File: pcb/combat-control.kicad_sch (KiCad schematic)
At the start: 0 parts

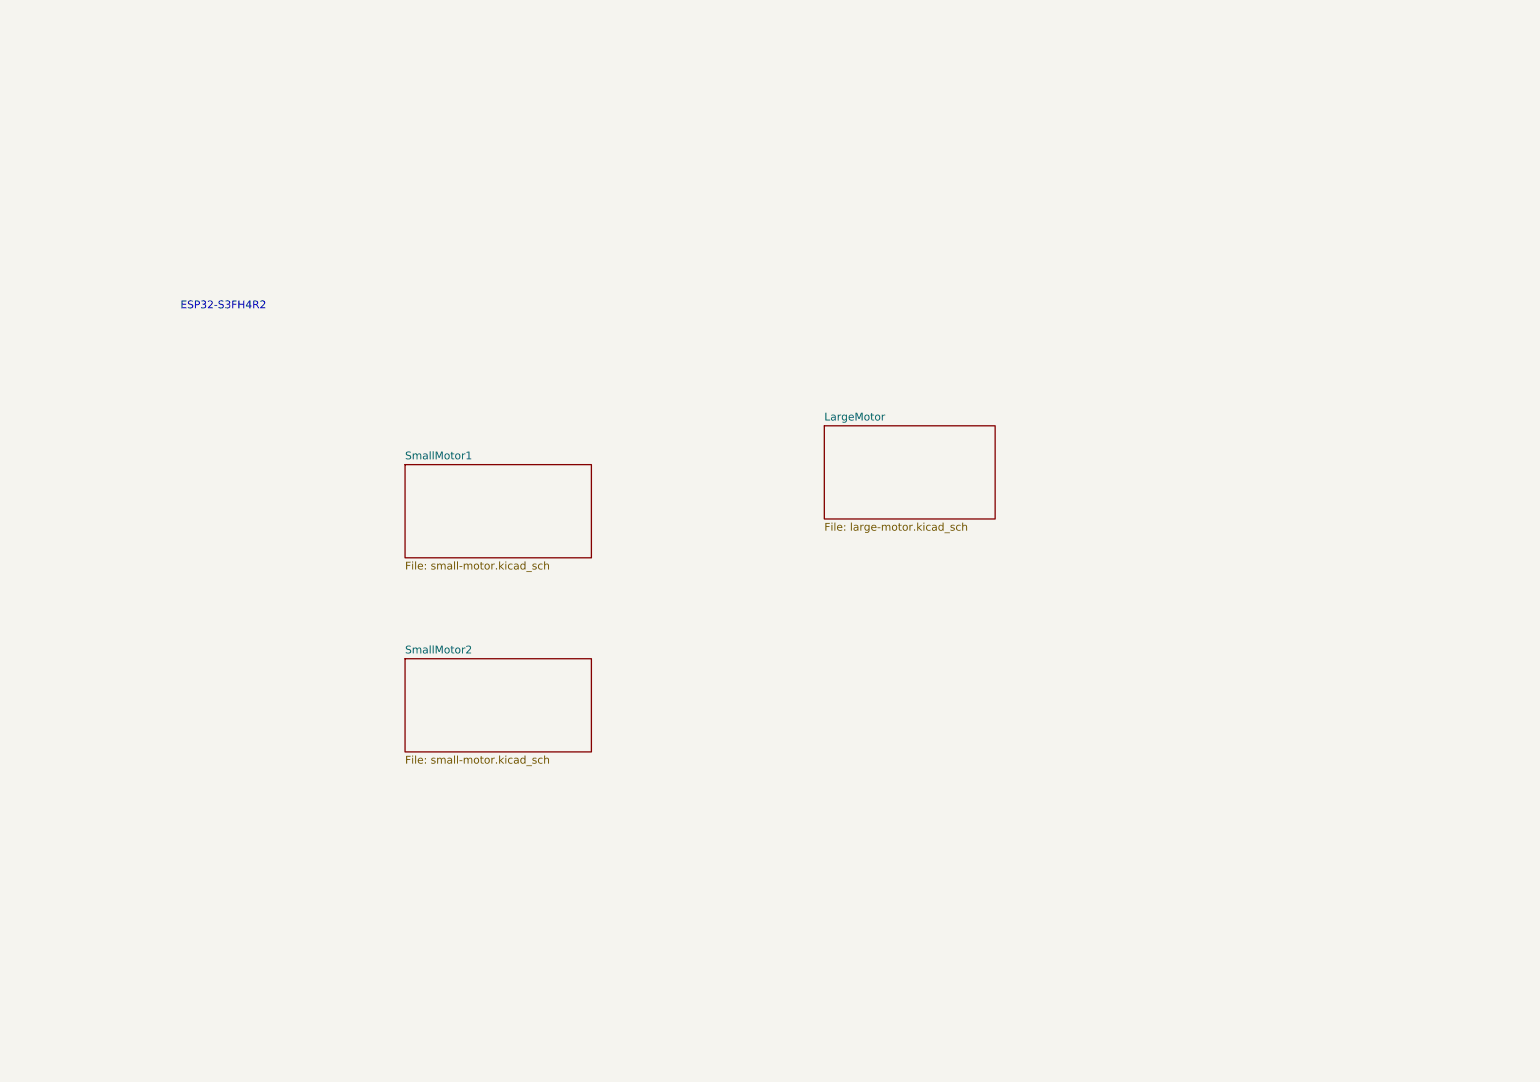
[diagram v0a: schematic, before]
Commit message: Save progress
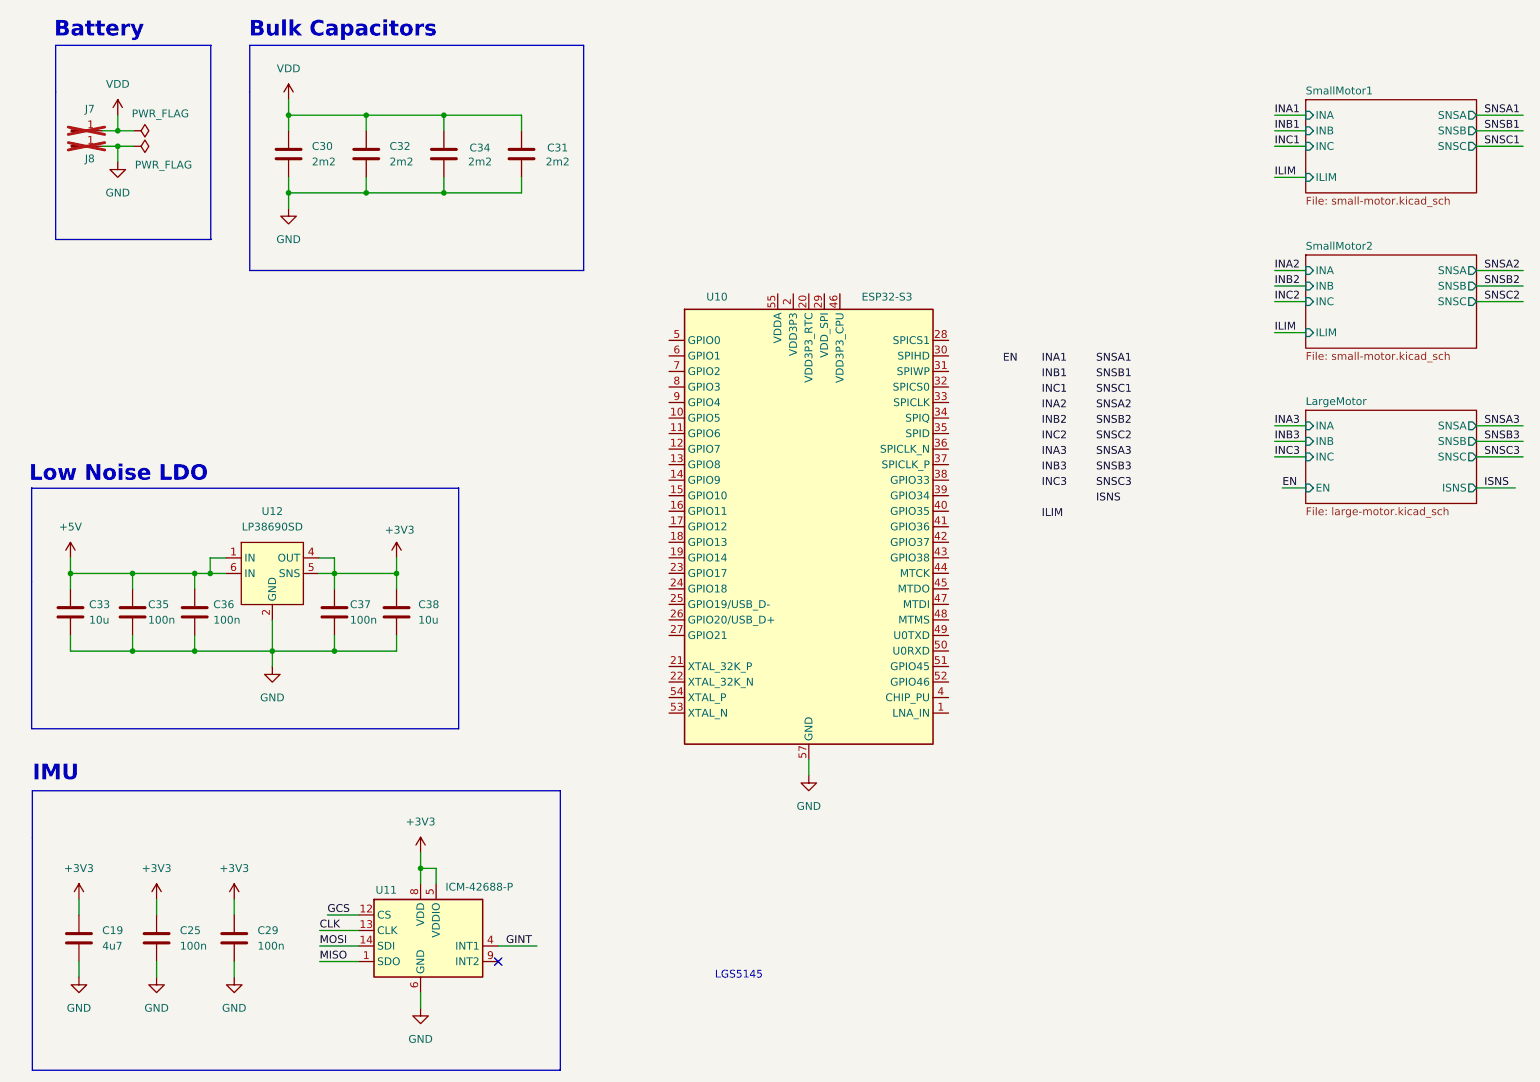
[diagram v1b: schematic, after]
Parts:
- added C19: 4u7, Capacitor_SMD:C_0402_1005Metric, symbol Device:C
- added C25, C29, C35, C36, C37: 100n, Capacitor_SMD:C_0402_1005Metric, symbol Device:C
- added C30, C31, C32, C34: 2m2, User_Footprints:C_D10xL16_Horizontal, symbol Device:C
- added C33: 10u, Capacitor_SMD:C_0603_1608Metric, symbol Device:C
- added C38: 10u, Capacitor_SMD:C_0402_1005Metric, symbol Device:C
- added J7, J8: Conn_01x01_Pin, MountingHole:MountingHole_3.2mm_M3_Pad_Via, symbol Connector:Conn_01x01_Pin
- added U10: ESP32-S3, Package_DFN_QFN:QFN-56-1EP_7x7mm_P0.4mm_EP4x4mm, symbol MCU_Espressif:ESP32-S3
- added U11: ICM-42688-P, Package_LGA:LGA-14_3x2.5mm_P0.5mm_LayoutBorder3x4y, symbol User_Symbols:ICM-42688-P
- added U12: LP38690SD, Package_DFN_QFN:DFN-6-1EP_3x3mm_P0.95mm_EP1.7x2.6mm, symbol User_Symbols:LP38690SD-3.3
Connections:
- new net: U10.2 (VDD3P3), U10.3 (VDD3P3)
- new net: U10.55 (VDDA), U10.56 (VDDA)
- new net +3V3: C19.1, C25.1, C29.1, C37.1, C38.1, U11.5 (VDDIO), U11.8 (VDD), U12.4 (OUT), U12.5 (SNS)
- new net +5V: C33.1, C35.1, C36.1, U12.1 (IN), U12.6 (IN)
- new net CLK: U11.13 (CLK)
- new net GCS: U11.12 (CS)
- new net GINT: U11.4 (INT1)
- new net GND: C19.2, C25.2, C29.2, C30.2, C31.2, C32.1, C33.2, C34.2, C35.2, C36.2, C37.2, C38.2, J8.1 (Pin_1), U10.57 (GND), U11.11 (RESV), U11.6 (GND), U11.7 (RESV), U12.2 (GND), U12.7 (PAD)
- new net MISO: U11.1 (SDO)
- new net MOSI: U11.14 (SDI)
- new net VDD: C30.1, C31.1, C32.2, C34.1, J7.1 (Pin_1)
- no-connect marks 0 -> 1
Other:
- sheet LargeMotor ports: added EN, INA, INB, INC, ISNS, SNSA, SNSB, SNSC; removed none
- sheet SmallMotor1 ports: added ILIM, INA, INB, INC, SNSA, SNSB, SNSC; removed none
- sheet SmallMotor2 ports: added ILIM, INA, INB, INC, SNSA, SNSB, SNSC; removed none
- note added: "Battery"
- note added: "Bulk Capacitors"
- note added: "IMU"
- note added: "LGS5145"
- note added: "Low Noise LDO"
- note removed: "ESP32-S3FH4R2"
